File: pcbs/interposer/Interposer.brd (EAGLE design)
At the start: 100 x 100 mm, 28 parts

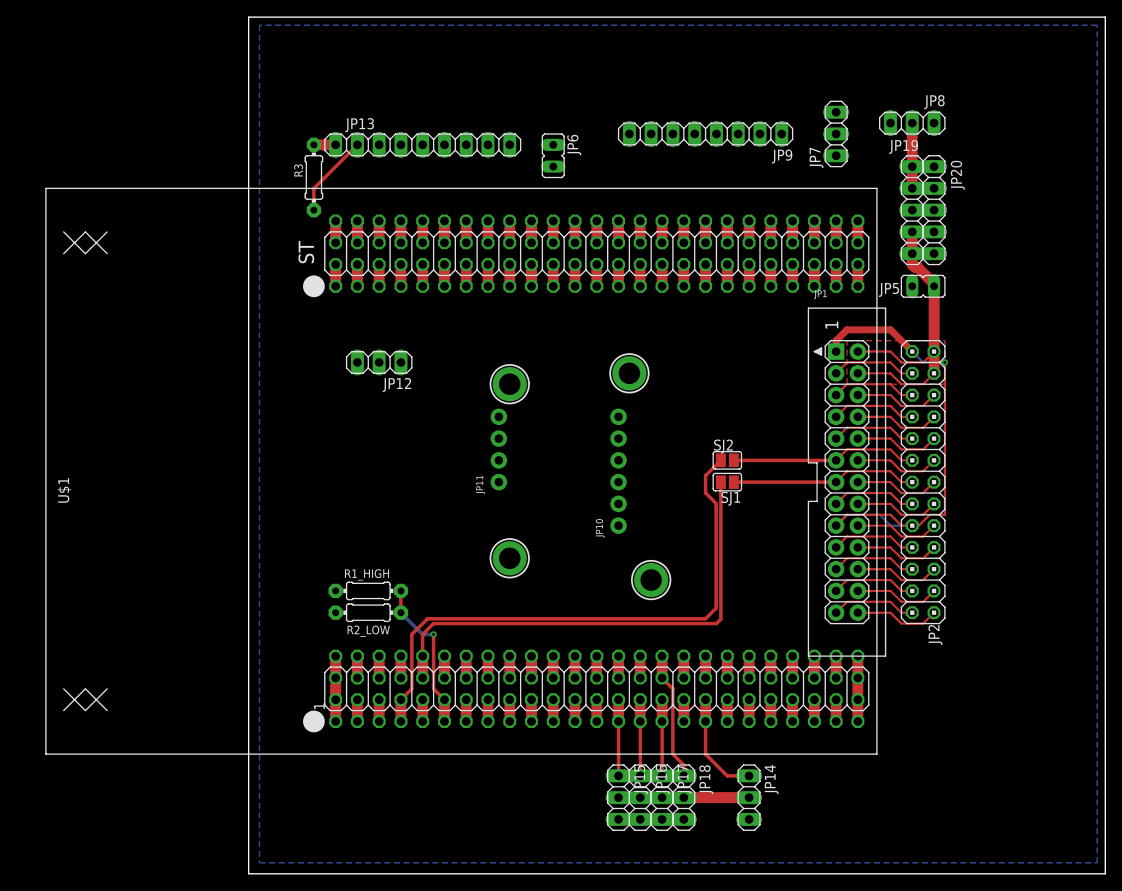
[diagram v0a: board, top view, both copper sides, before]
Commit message: Finished interposer board.
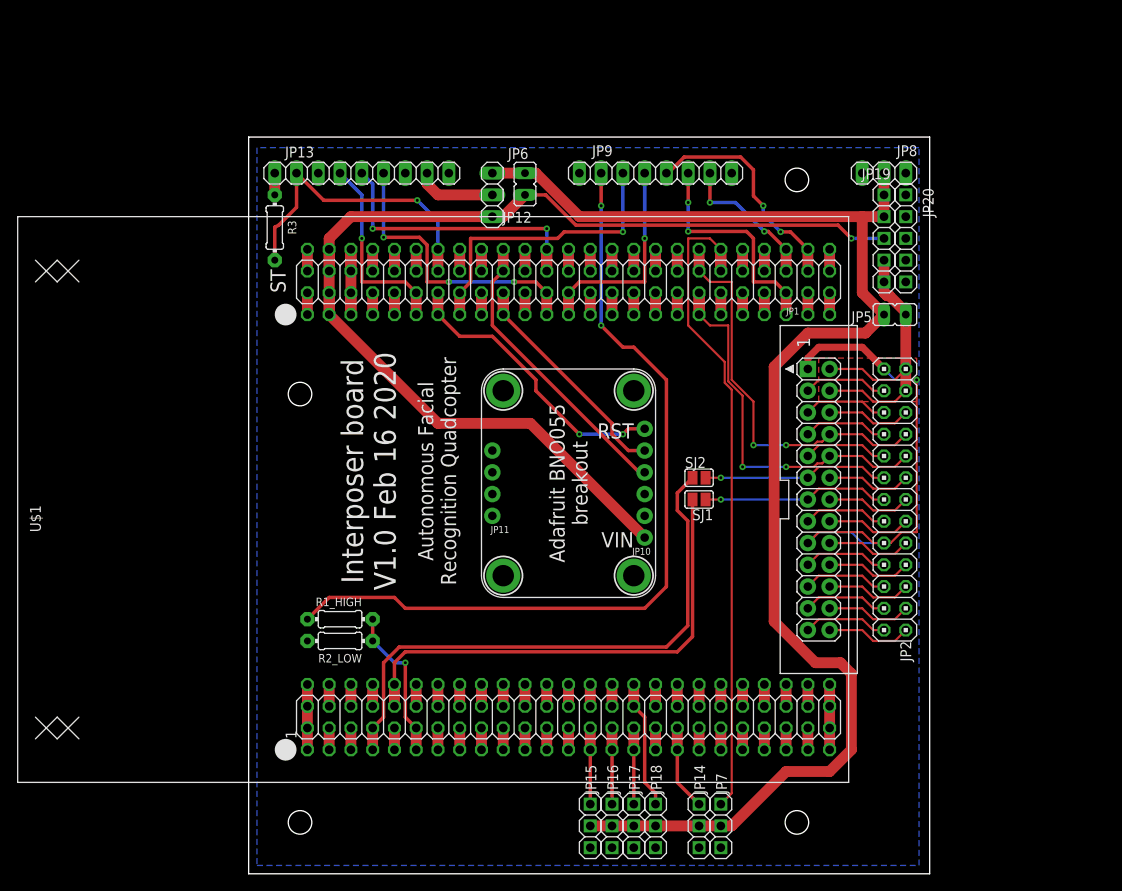
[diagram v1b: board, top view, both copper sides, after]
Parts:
- added U$2, U$3, U$4, U$5: (no value), HighCurrentTransistorAndDriver:RPI_MOUNTING_HOLE
- JP12: value GPS_5Vsrc_sel -> GPS_5Vsrc
- JP14, JP15, JP16, JP17, JP18, JP7: device pinhead:1X03 -> Interposer:1X03
- JP19, JP20: device pinhead:1X05 -> Interposer:1X05
- JP6: value (none) -> STM_PWR
- moved JP7 81.9 mm to (55.1, 5.59), turned to 270 degrees
- moved U$31 28.0 mm to (29.7, 56.4), turned to 90 degrees
- moved JP12 23.6 mm to (28.4, 79.2), turned to 270 degrees
- moved U$29 22.4 mm to (29.7, 34.8), turned to 90 degrees
- moved U$32 14.6 mm to (45.0, 34.8), turned to 90 degrees
- moved JP13 7.84 mm to (13.2, 81.8)
- moved R3 7.42 mm to (3.05, 75.4)
- moved JP9 7.42 mm to (47.5, 81.8)
- moved JP14 6.71 mm to (52.6, 5.59)
- moved JP8 6.71 mm to (74.2, 81.8)
- moved JP20 4.67 mm to (76.7, 74.2)
- moved R1_HIGH 4.67 mm to (10.7, 29.7)
- moved JP6 4.67 mm to (32.3, 80.5)
- moved R2_LOW 4.67 mm to (10.7, 27.2)
- moved U$1 4.67 mm to (6.86, 17.0)
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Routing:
- net +5V: track 22.9 -> 165.1 mm
- net STM5V: track 0.00 -> 125.5 mm, vias 0 -> 1
- net BAT+: track 0.00 -> 96.7 mm, vias 0 -> 2
- net CAM_SERVO: track 0.00 -> 75.5 mm
- net RPI_TXD: track 9.94 -> 46.3 mm, vias 0 -> 2
- net ESTOP_L: track 0.00 -> 34.4 mm, vias 0 -> 1
- net RPI_RXD: track 9.94 -> 44.3 mm, vias 0 -> 2
- net BNO_SDA: track 0.00 -> 34.3 mm
- net GPS_RX: track 0.00 -> 34.3 mm, vias 0 -> 3
- net BNO_RST_L: track 0.00 -> 33.5 mm, vias 0 -> 2
- net GPS_TX: track 0.00 -> 32.3 mm, vias 0 -> 2
- net ESC3: track 0.00 -> 26.7 mm, vias 0 -> 2
- net ESC2: track 0.00 -> 26.7 mm, vias 0 -> 2
- net BNO_SCL: track 0.00 -> 26.4 mm
- net GPS_EN: track 9.72 -> 36.0 mm, vias 0 -> 1
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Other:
- board size 100 x 100 mm -> 79.5 x 86 mm
- board text added: "Adafruit BNO055 breakout"
- board text added: "Autonomous Facial Recognition Quadcopter"
- board text added: "Interposer board V1.0 Feb 16 2020"
- board text added: "RST"
- board text added: "VIN"
